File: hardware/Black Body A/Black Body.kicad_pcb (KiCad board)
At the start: 2 copper layers, 52 x 53.8 mm, 42 parts, among them IC2 MCP96L00T-E_MX, J1 53307-2471, J2 Conn_01x02, J4 LogicAnalyzer, J5 Conn_02x04_Top_Bottom, J7 Conn_02x03_Top_Bottom

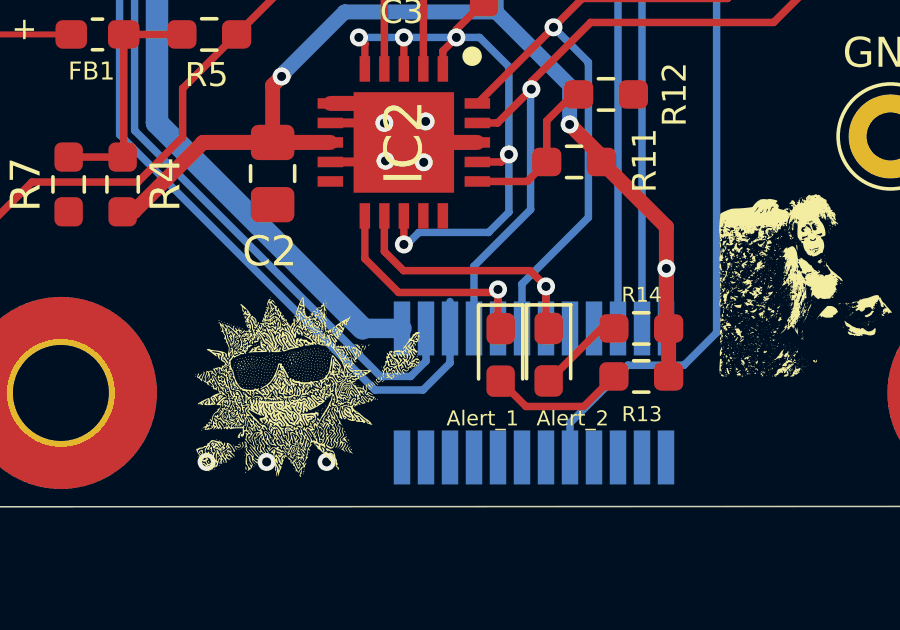
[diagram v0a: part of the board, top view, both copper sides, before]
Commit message: updated step file
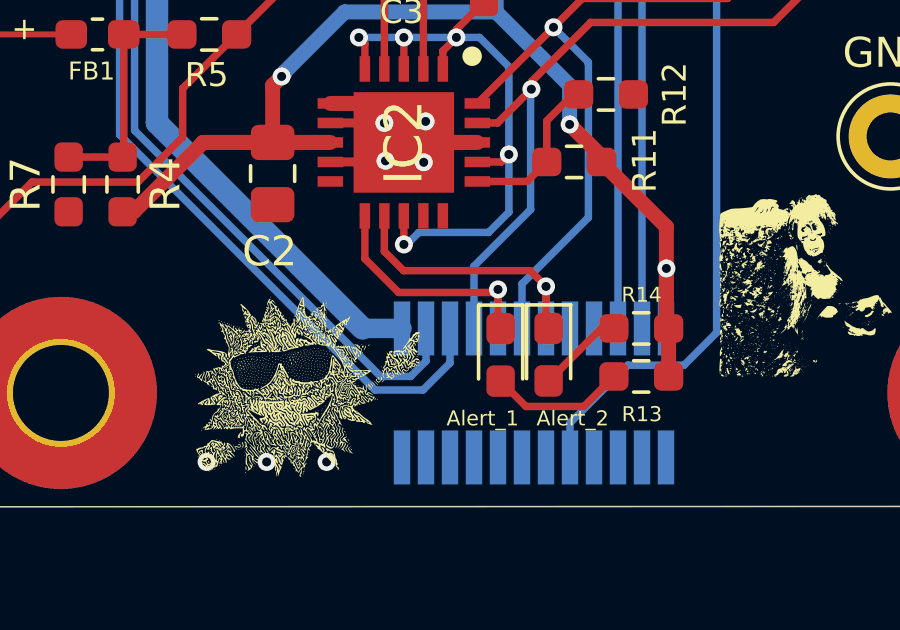
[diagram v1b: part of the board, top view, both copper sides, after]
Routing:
- net /CAN_L: track 35.8 -> 34.9 mm
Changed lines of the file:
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@@
-	)
-	(segment
-		(start 108.1125 114.8)
-		(end 108.1125 113.904202)
-		(width 0.25)
-		(layer "B.Cu")
-		(net 38)
 	)
 	(segment
